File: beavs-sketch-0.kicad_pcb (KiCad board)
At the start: 4 copper layers, 74 x 74 mm, 56 parts, among them J1 USB_C_Receptacle_USB2.0_16P, J10 Conn_01x03, J11 Conn_01x03, J12 Micro_SD_Card, J2 Conn_Coaxial, J3 Conn_01x02, J4 Conn_Coaxial, J5 Conn_01x02, J6 Conn_01x03, J7 Conn_01x03, J8 Conn_01x03, J9 Conn_01x03, Q2 SiS427EDN, U1 RP2040, U10 INA745A, U11 INA745A, U12 INA745A, U13 INA745A, U14 ISM6HG256X, U15 SN74LVC8T245, U2 W25Q128JVS, U3 MS5607-02BA, U4 RFM95W-915S2, U5 MAX-M10S, U6 INA745A, U7 AMS1117-3.3, U8 AMS1117-5.0, U9 INA745A, Y1 Crystal_GND24

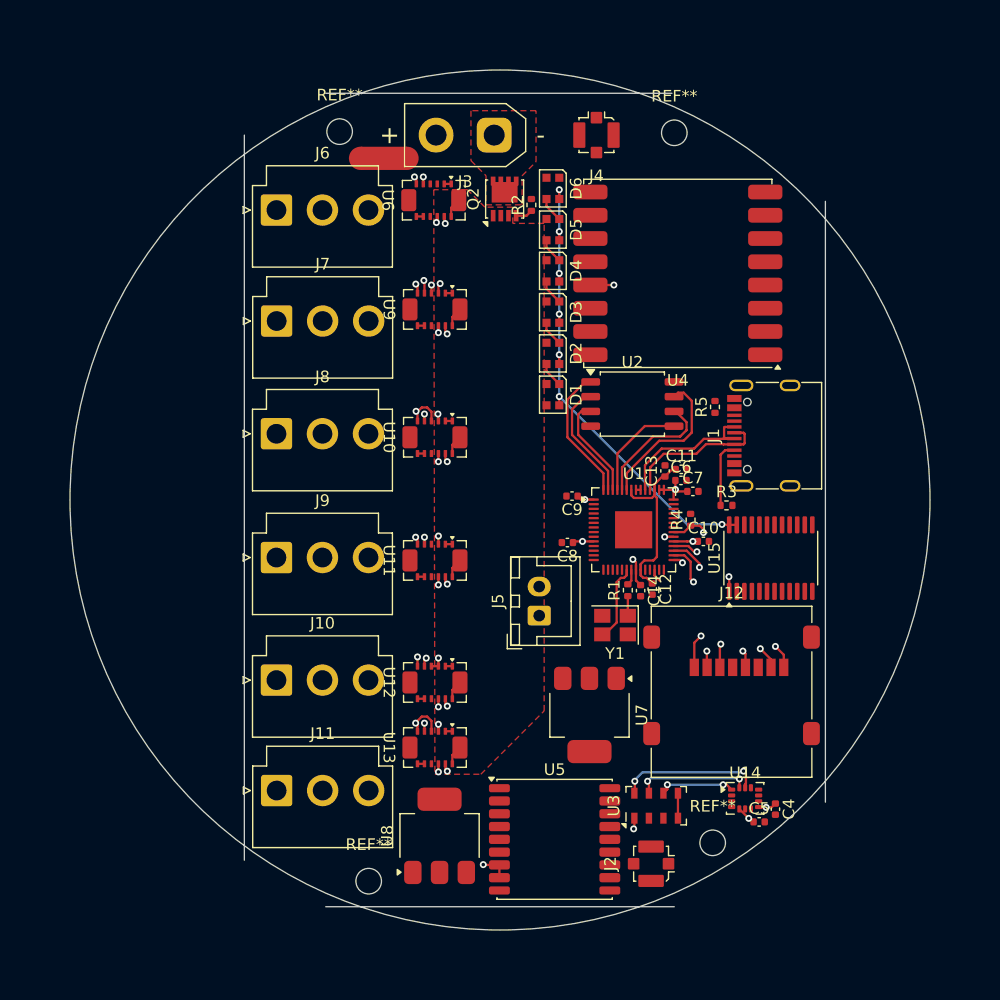
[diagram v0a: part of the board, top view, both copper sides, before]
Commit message: add 3d models and do other stuff
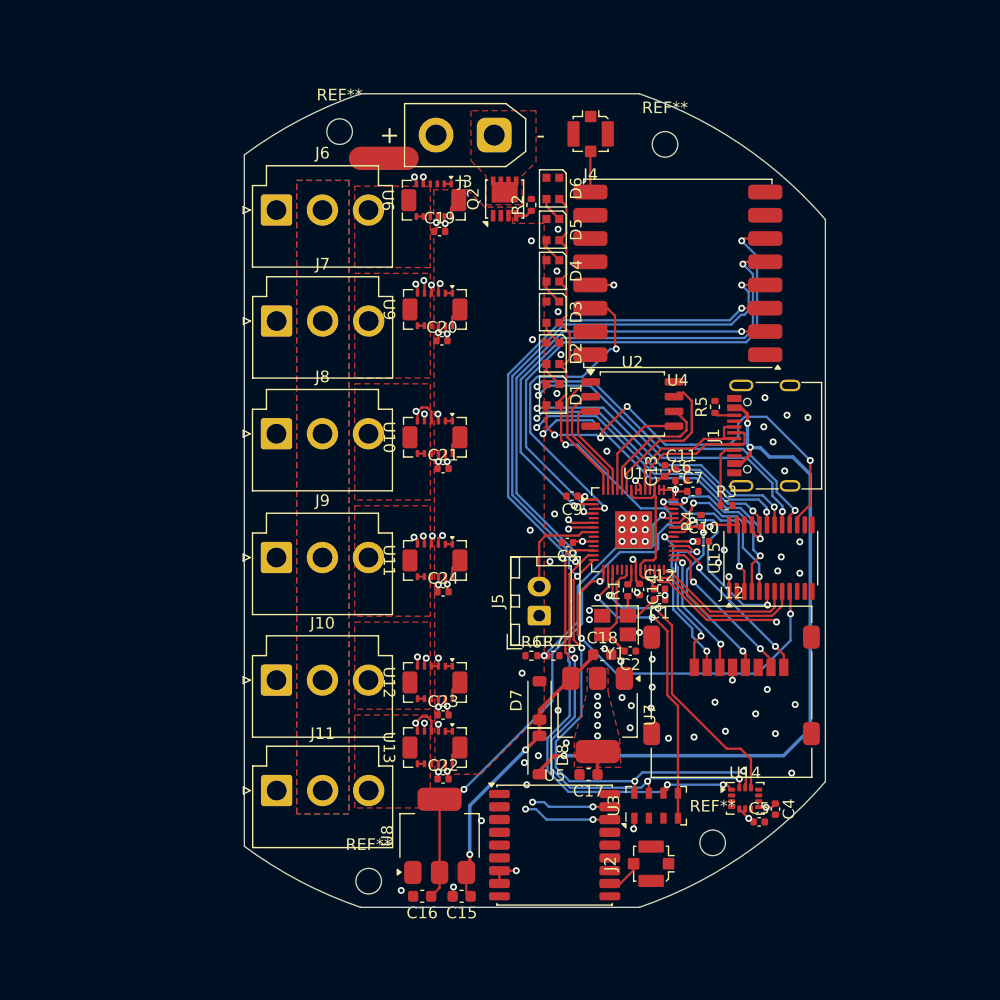
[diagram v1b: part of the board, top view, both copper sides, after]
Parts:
- added C1: C_Small, Capacitor_SMD:C_0402_1005Metric, F.Cu at (212.7, 96.6)
- added C15: 10u, Capacitor_SMD:C_0603_1608Metric, F.Cu at (195.7, 122.1)
- added C16: 22u, Capacitor_SMD:C_0603_1608Metric, F.Cu at (192.3, 122.1)
- added C17: 22u, Capacitor_SMD:C_0603_1608Metric, F.Cu at (206.6, 111.6)
- added C18: 10u, Capacitor_SMD:C_0603_1608Metric, F.Cu at (207.8, 101.3)
- added C19: 100n, Capacitor_SMD:C_0402_1005Metric, F.Cu at (193.8, 64.9)
- added C2: C_Small, Capacitor_SMD:C_0402_1005Metric, F.Cu at (210.2, 101.0)
- added C20: 100n, Capacitor_SMD:C_0402_1005Metric, F.Cu at (194.0, 74.3)
- added C21: 100n, Capacitor_SMD:C_0402_1005Metric, F.Cu at (194.1, 85.3)
- added C22: 100n, Capacitor_SMD:C_0402_1005Metric, F.Cu at (194.1, 112.0)
- added C23: 100n, Capacitor_SMD:C_0402_1005Metric, F.Cu at (194.1, 106.5)
- added C24: 100n, Capacitor_SMD:C_0402_1005Metric, F.Cu at (194.1, 95.9)
- added D7: D_Schottky, Diode_SMD:D_SOD-123, F.Cu at (202.4, 105.2)
- added D8: D_Schottky, Diode_SMD:D_SOD-123, F.Cu at (202.4, 110.0)
- added R6: R_Small, Resistor_SMD:R_0402_1005Metric, F.Cu at (201.7, 101.4)
- added R7: R_Small, Resistor_SMD:R_0402_1005Metric, F.Cu at (203.6, 101.4)
- J10, J11, J6, J7, J8, J9: footprint Connector_JST:JST_VH_B3P-VH-B_1x03_P3.96mm_Vertical -> beavs-footprints:JST_VH_B3P-VH-B_1x03_P3.96mm_Vertical_model
- moved REF** 1.28 mm to (213.2, 57.4)
- moved R4 0.91 mm to (216.3, 89.8)
- moved U7 0.70 mm to (207.4, 106.5)
- moved C12 0.62 mm to (212.7, 95.7), turned to 0 degrees
- moved J4 0.51 mm to (206.8, 56.5)
- moved U5 0.50 mm to (203.7, 117.7)
- moved C14 0.14 mm to (211.0, 95.7)
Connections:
- net Net-(J1-VBUS-PadA4) renamed VBUS
- D1 pad 3: unconnected-(D1-DIN-Pad3) -> Net-(D1-DIN)
- J10 pad 1: unconnected-(J10-Pin_1-Pad1) -> /servos/S5
- J11 pad 1: unconnected-(J11-Pin_1-Pad1) -> /servos/S6
- J5 pad 1: /ARM_SWITCH -> GND
- J5 pad 2: GND -> /ARM_SWITCH
- J6 pad 1: unconnected-(J6-Pin_1-Pad1) -> /servos/S1
- J7 pad 1: unconnected-(J7-Pin_1-Pad1) -> /servos/S2
- J8 pad 1: unconnected-(J8-Pin_1-Pad1) -> /servos/S3
- J9 pad 1: unconnected-(J9-Pin_1-Pad1) -> /servos/S4
- U1 pad 12: unconnected-(U1-GPIO9-Pad12) -> /Radio/MOSI
- U1 pad 13: unconnected-(U1-GPIO10-Pad13) -> /Radio/MISO
- U1 pad 14: unconnected-(U1-GPIO11-Pad14) -> /Radio/SCK
- U1 pad 15: unconnected-(U1-GPIO12-Pad15) -> /mcu/M_LED_D
- U1 pad 16: unconnected-(U1-GPIO13-Pad16) -> /Sensors/BARO_CS
- U1 pad 17: unconnected-(U1-GPIO14-Pad17) -> /Sensors/IMU_CS
- U1 pad 2: unconnected-(U1-GPIO0-Pad2) -> /Radio/CS
- U1 pad 27: unconnected-(U1-GPIO16-Pad27) -> /mcu/M_S6
- U1 pad 28: unconnected-(U1-GPIO17-Pad28) -> /mcu/M_S5
- U1 pad 3: unconnected-(U1-GPIO1-Pad3) -> /Radio/D0
- U1 pad 36: unconnected-(U1-GPIO24-Pad36) -> /mcu/M_S4
- U1 pad 37: unconnected-(U1-GPIO25-Pad37) -> /mcu/M_S3
- U1 pad 38: unconnected-(U1-GPIO26_ADC0-Pad38) -> /mcu/BATTERY_SENSE
- U1 pad 4: unconnected-(U1-GPIO2-Pad4) -> /Radio/RESET
- U1 pad 40: unconnected-(U1-GPIO28_ADC2-Pad40) -> /mcu/M_S1
- U1 pad 41: unconnected-(U1-GPIO29_ADC3-Pad41) -> /mcu/M_S2
- U1 pad 6: unconnected-(U1-GPIO4-Pad6) -> /Sensors/SDA
- U1 pad 7: unconnected-(U1-GPIO5-Pad7) -> /Sensors/SCL
- U1 pad 8: unconnected-(U1-GPIO6-Pad8) -> /ARM_SWITCH
- U10 pad 4: /servos/SCL -> /Sensors/SCL
- U10 pad 5: /servos/SDA -> /Sensors/SDA
- U10 pad 6: /servos/SCL -> /Sensors/SCL
- U11 pad 5: /servos/SDA -> /Sensors/SDA
- U11 pad 6: /servos/SCL -> /Sensors/SCL
- U12 pad 5: /servos/SDA -> /Sensors/SDA
- U12 pad 6: /servos/SCL -> /Sensors/SCL
- U13 pad 4: /servos/SCL -> /Sensors/SCL
- U13 pad 5: /servos/SDA -> /Sensors/SDA
- U13 pad 6: /servos/SCL -> /Sensors/SCL
- U14 pad 1: /Sensors/MISO -> /Radio/MISO
- U14 pad 13: /Sensors/SCK -> /Radio/SCK
- U14 pad 14: /Sensors/MOSI -> /Radio/MOSI
- U15 pad 15: unconnected-(U15-B7-Pad15) -> Net-(D1-DIN)
- U15 pad 16: unconnected-(U15-B6-Pad16) -> /servos/S6
- U15 pad 17: unconnected-(U15-B5-Pad17) -> /servos/S5
- U15 pad 18: unconnected-(U15-B4-Pad18) -> /servos/S4
- U15 pad 19: unconnected-(U15-B3-Pad19) -> /servos/S3
- U15 pad 20: unconnected-(U15-B2-Pad20) -> /servos/S2
- U15 pad 21: unconnected-(U15-B1-Pad21) -> /servos/S1
- U15 pad 3: unconnected-(U15-A1-Pad3) -> /mcu/M_S1
- U15 pad 4: unconnected-(U15-A2-Pad4) -> /mcu/M_S2
- U15 pad 5: unconnected-(U15-A3-Pad5) -> /mcu/M_S3
- U15 pad 6: unconnected-(U15-A4-Pad6) -> /mcu/M_S4
- U15 pad 7: unconnected-(U15-A5-Pad7) -> /mcu/M_S5
- U15 pad 8: unconnected-(U15-A6-Pad8) -> /mcu/M_S6
- U15 pad 9: unconnected-(U15-A7-Pad9) -> /mcu/M_LED_D
- U3 pad 6: /Sensors/MISO -> /Radio/MISO
- U3 pad 7: /Sensors/MOSI -> /Radio/MOSI
- U3 pad 8: /Sensors/SCK -> /Radio/SCK
- U4 pad 14: unconnected-(U4-DIO0-Pad14) -> /Radio/D0
- U4 pad 2: unconnected-(U4-MISO-Pad2) -> /Radio/MISO
- U4 pad 3: unconnected-(U4-MOSI-Pad3) -> /Radio/MOSI
- U4 pad 4: unconnected-(U4-SCK-Pad4) -> /Radio/SCK
- U4 pad 5: unconnected-(U4-NSS-Pad5) -> /Radio/CS
- U4 pad 6: unconnected-(U4-RESET-Pad6) -> /Radio/RESET
- U6 pad 5: /servos/SDA -> /Sensors/SDA
- U6 pad 6: /servos/SCL -> /Sensors/SCL
- U7 pad 1: unconnected-(U7-GND-Pad1) -> GND
- U7 pad 2: unconnected-(U7-VO-Pad2) -> +3V3
- U7 pad 3: unconnected-(U7-VI-Pad3) -> Net-(D7-K)
- U8 pad 1: unconnected-(U8-GND-Pad1) -> GND
- U8 pad 2: unconnected-(U8-VO-Pad2) -> +5V
- U8 pad 3: unconnected-(U8-VI-Pad3) -> Net-(D7-K)
- U9 pad 5: /servos/SDA -> /Sensors/SDA
- U9 pad 6: /servos/SCL -> /Sensors/SCL
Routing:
- net /Sensors/SCL: track 0.00 -> 95.2 mm, vias 0 -> 9
- net /Sensors/SDA: track 0.00 -> 91.8 mm, vias 0 -> 9
- net /Radio/SCK: track 0.00 -> 86.3 mm, vias 0 -> 5
- net /servos/S6: track 0.00 -> 86.3 mm, vias 0 -> 3
- net /Radio/MOSI: track 0.00 -> 83.8 mm, vias 0 -> 5
- net /Radio/MISO: track 0.00 -> 80.0 mm, vias 0 -> 5
- net /servos/S5: track 0.00 -> 75.4 mm, vias 0 -> 3
- net /servos/S1: track 0.00 -> 66.0 mm, vias 0 -> 3
- net VBUS: track 0.00 -> 59.8 mm, vias 0 -> 3
- net /servos/S4: track 0.00 -> 59.1 mm, vias 0 -> 3
- net /servos/SCL: track 57.0 -> 0.00 mm, vias 6 -> 0
- net /servos/S2: track 0.00 -> 54.9 mm, vias 0 -> 3
- net /servos/SDA: track 51.5 -> 0.00 mm, vias 6 -> 0
- net /servos/S3: track 0.00 -> 49.2 mm, vias 0 -> 2
- net /Radio/RESET: track 0.00 -> 46.3 mm, vias 0 -> 2
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- added copper zone on F.Cu, net +3V3
- added copper zone on B.Cu, net GND1
- added copper zone on F.Cu, net GND1
- added copper zone on F.Cu, net Net-(J10-Pin_3)
- added copper zone on F.Cu, net Net-(J11-Pin_3)
- added copper zone on F.Cu, net Net-(J6-Pin_3)
- added copper zone on F.Cu, net Net-(J7-Pin_3)
- added copper zone on F.Cu, net Net-(J8-Pin_3)
- added copper zone on F.Cu, net Net-(J9-Pin_3)
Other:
- board size 74 x 74 mm -> 50 x 70 mm
